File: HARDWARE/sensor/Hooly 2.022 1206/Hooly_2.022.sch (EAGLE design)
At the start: 36 parts, among them IC2 MCP1703CB, Q1 8MHz Crystal, U3 MCP73831, U5 ATMEGA328P-AU

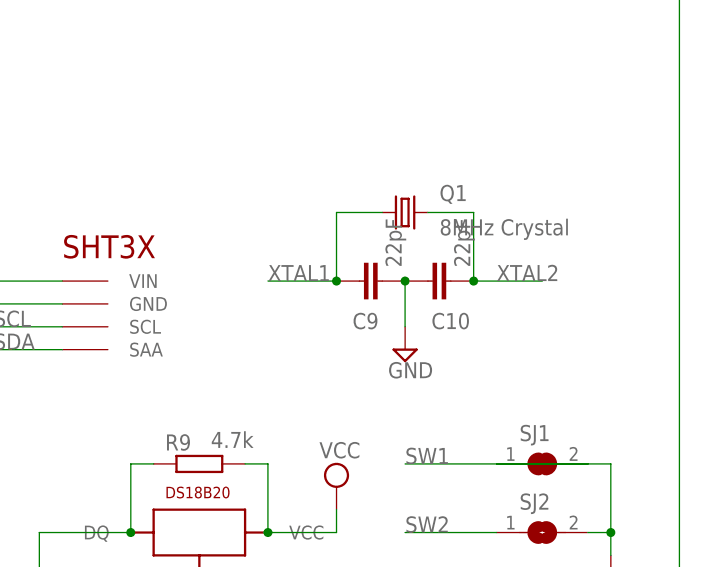
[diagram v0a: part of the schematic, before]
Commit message: Hardware update
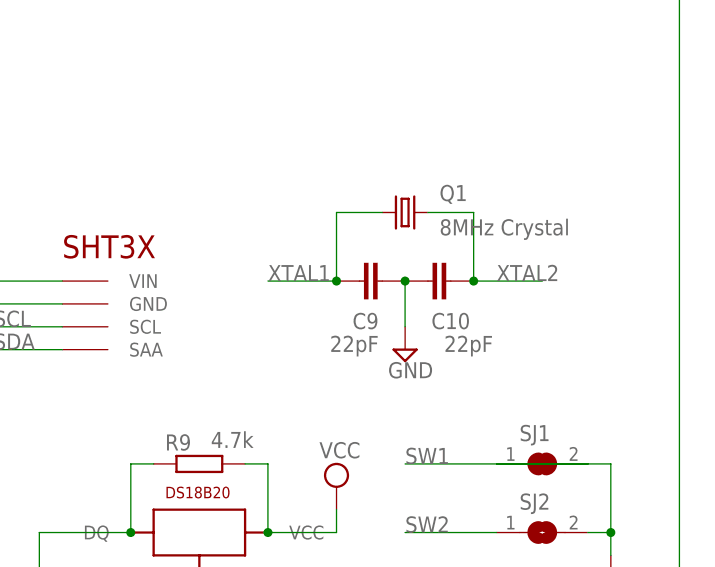
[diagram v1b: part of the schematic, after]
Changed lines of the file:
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@@
 <classes>
 <class number="0" name="default" width="0" drill="0">
+<clearance class="0" value="0.508"/>
 </class>
 </classes>
@@
 <instance part="C9" gate="G$1" x="119.38" y="109.22" smashed="yes" rot="R90">
 <attribute name="NAME" x="121.539" y="105.664" size="1.778" layer="95" rot="R180"/>
-<attribute name="VALUE" x="124.079" y="110.744" size="1.778" layer="96" rot="R90"/>
+<attribute name="VALUE" x="121.539" y="103.124" size="1.778" layer="96" rot="R180"/>
 </instance>
 <instance part="C10" gate="G$1" x="127" y="109.22" smashed="yes" rot="R90">
 <attribute name="NAME" x="131.699" y="105.664" size="1.778" layer="95" rot="R180"/>
-<attribute name="VALUE" x="131.699" y="110.744" size="1.778" layer="96" rot="R90"/>
+<attribute name="VALUE" x="134.239" y="103.124" size="1.778" layer="96" rot="R180"/>
 </instance>
 </instances>
